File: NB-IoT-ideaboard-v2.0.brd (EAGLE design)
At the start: 74.8 x 54.5 mm, 102 parts, among them Q1 32.768kHz, Q2 8MHz, Q3 9013, Q4 9013, Q5 9013, U1 STM32F103RBT6, U2 MCP73831T-2ACI/OT, U3 AP2112-3.3, U4 PAM2401, U5 MICROSIM, U6 BC92

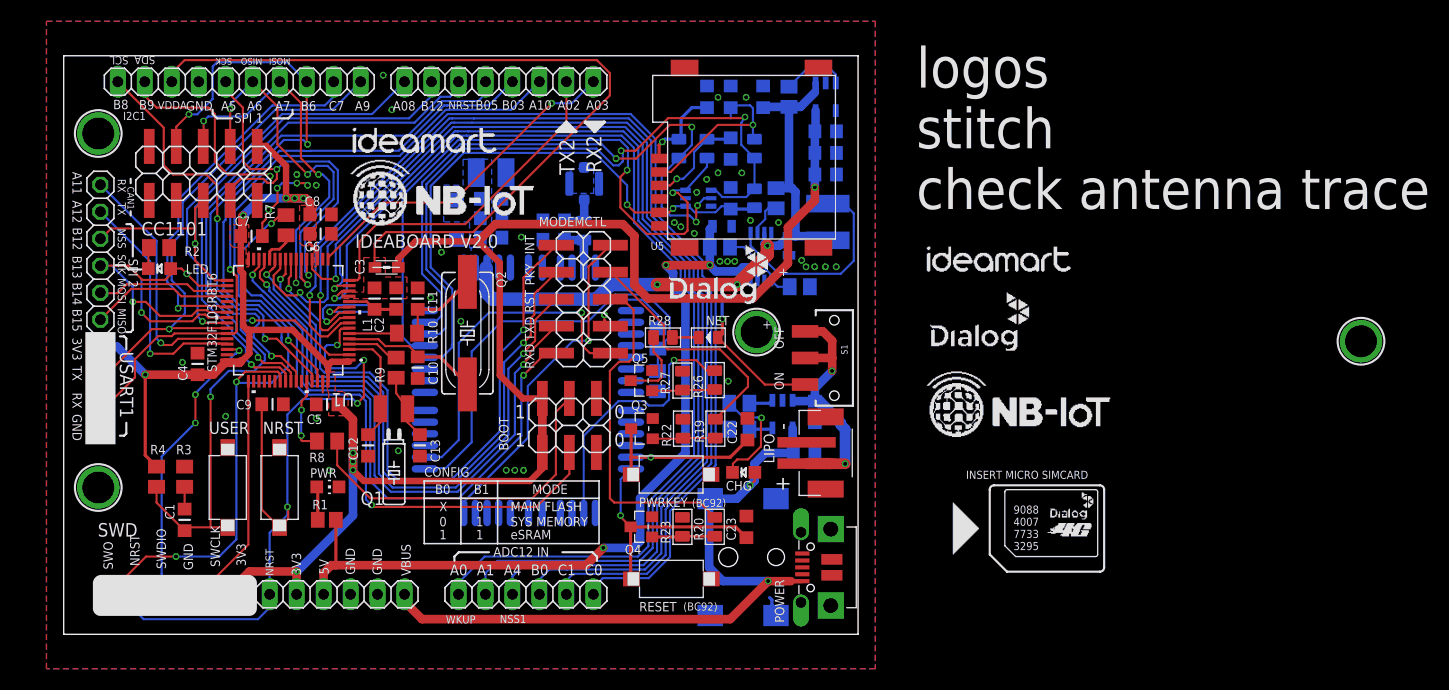
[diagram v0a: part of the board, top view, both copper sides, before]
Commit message: Minor changes
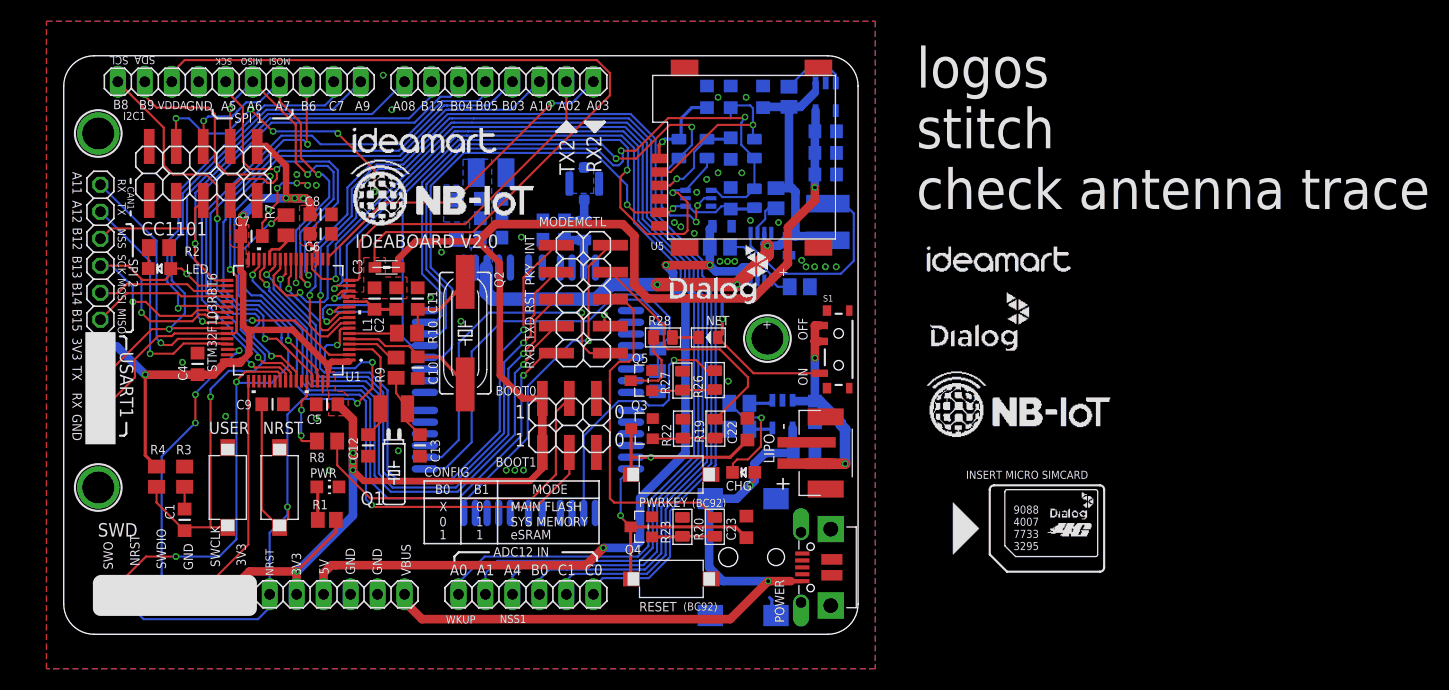
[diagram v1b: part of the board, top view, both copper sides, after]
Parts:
- removed $H4: MOUNTINGHOLE3.0THIN, Adafruit SIM808 Breakout:MOUNTINGHOLE_3.0_PLATEDTHIN
- R1: value 1k -> 330R
- R13, R28: value 2.2k -> 2k2
- R19, R20, R26: value 4.7k -> 4k7
- R25: value 2.2k -> 0R
- R6: value 5.6k -> 5k7
- S1: device SparkFun-Electromechanical:SWITCH-SPDT-SMD -> SparkFun-Electromechanical:SWITCH-SPST-SMD-A
- moved $H1 1.18 mm to (217.4, 26.2)
- moved S1 0.91 mm to (224.1, 25.2)
- moved Q2 0.20 mm to (189.0, 26.7)
- renumbered ANT1 to RF_ANT
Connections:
- net +3V3: now also R1.2
- net +5V: no longer R1.2
- net PA4: now also CC1101.4
- net PB6: no longer CC1101.4
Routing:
- net PA4: track 99.7 -> 128.2 mm, vias 1 -> 6
- net PB6: track 58.6 -> 39.4 mm, vias 3 -> 2
- net +3V3: track 206.5 -> 212.9 mm
- net +5V: track 79.7 -> 75.5 mm
- net +4.1V: track 26.7 -> 23.0 mm
- net PC1: track 102.7 -> 104.2 mm
- net PC0: track 103.0 -> 104.5 mm
- net PB0: track 106.1 -> 107.6 mm
- net V+: track 76.0 -> 76.9 mm
- net JNTRST: track 50.4 -> 51.3 mm
- net NRST: track 69.6 -> 70.5 mm
- net PA8: track 39.0 -> 39.8 mm
- net PB12: track 50.5 -> 51.2 mm
- net PB5: track 52.3 -> 53.0 mm
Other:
- outline, holes or cut-outs redrawn
- board text added: "2020/11/01"
- board text added: "B04"
- board text added: "BOOT0"
- board text added: "BOOT1"
- board text removed: "2018/06/01"
